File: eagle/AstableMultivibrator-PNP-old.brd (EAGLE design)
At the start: 30.5 x 15.2 mm, 10 parts, among them T1 BC557, T2 BC557

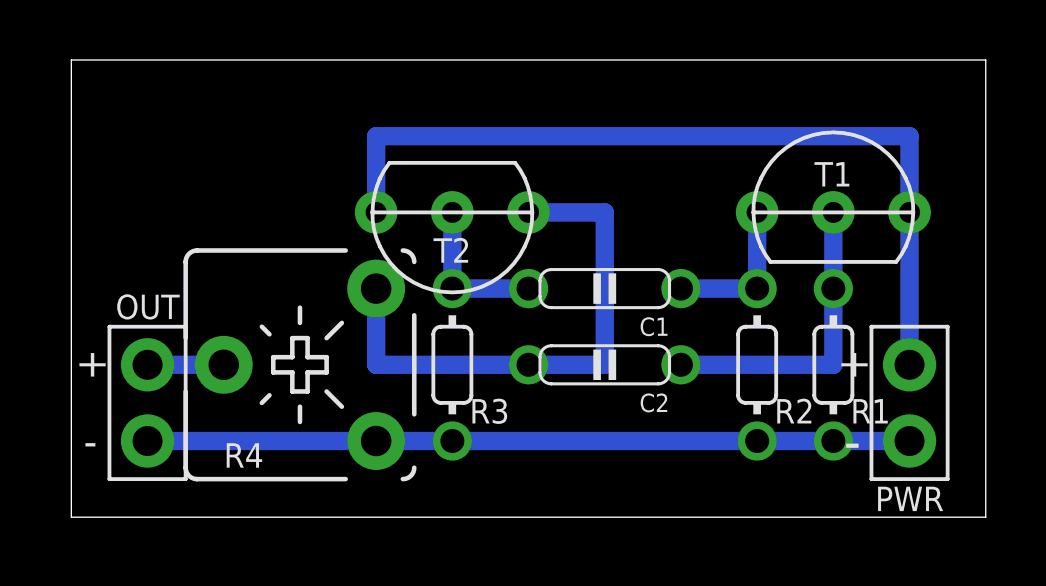
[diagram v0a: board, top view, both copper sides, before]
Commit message: ...
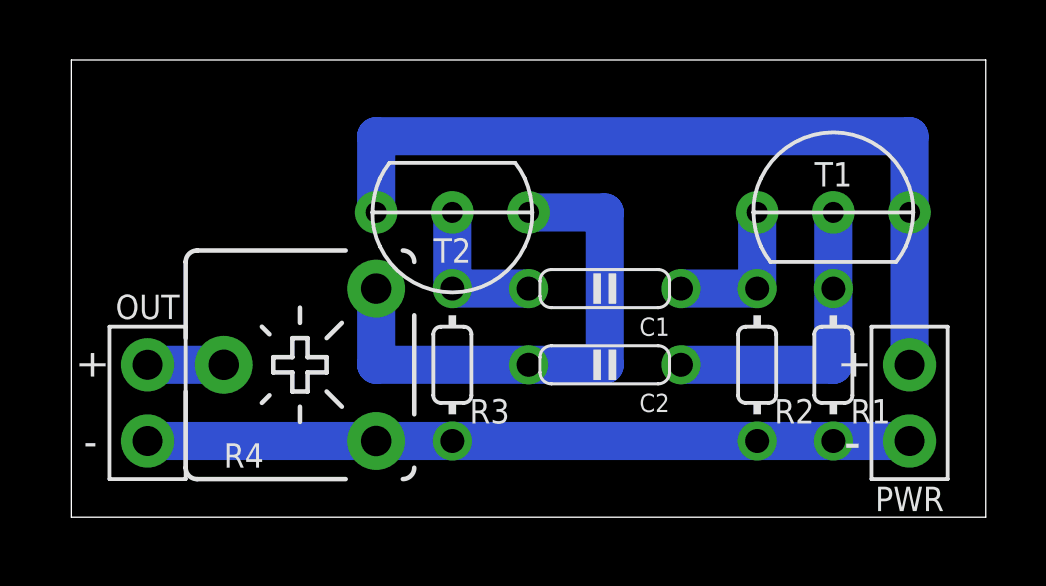
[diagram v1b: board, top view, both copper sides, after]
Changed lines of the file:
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@@
 <contactref element="C1" pad="1"/>
 <contactref element="R2" pad="2"/>
-<wire x1="20.32" y1="7.62" x2="22.86" y2="7.62" width="0.6096" layer="16"/>
-<wire x1="22.86" y1="7.62" x2="22.86" y2="10.16" width="0.6096" layer="16"/>
+<wire x1="20.32" y1="7.62" x2="22.86" y2="7.62" width="1.27" layer="16"/>
+<wire x1="22.86" y1="7.62" x2="22.86" y2="10.16" width="1.27" layer="16"/>
 <wire x1="22.86" y1="10.16" x2="22.86" y2="7.62" width="0" layer="19" extent="1-1"/>
 </signal>
@@
 <contactref element="C1" pad="2"/>
 <contactref element="R3" pad="2"/>
-<wire x1="15.24" y1="7.62" x2="12.7" y2="7.62" width="0.6096" layer="16"/>
-<wire x1="12.7" y1="7.62" x2="12.7" y2="10.16" width="0.6096" layer="16"/>
+<wire x1="15.24" y1="7.62" x2="12.7" y2="7.62" width="1.27" layer="16"/>
+<wire x1="12.7" y1="7.62" x2="12.7" y2="10.16" width="1.27" layer="16"/>
 </signal>
 <signal name="N$1">
@@
 <contactref element="C2" pad="2"/>
 <contactref element="R4" pad="E"/>
-<wire x1="15.24" y1="5.08" x2="10.16" y2="5.08" width="0.6096" layer="16"/>
-<wire x1="10.16" y1="5.08" x2="10.16" y2="7.62" width="0.6096" layer="16"/>
-<wire x1="15.24" y1="10.16" x2="17.78" y2="10.16" width="0.6096" layer="16"/>
-<wire x1="17.78" y1="10.16" x2="17.78" y2="5.08" width="0.6096" layer="16"/>
-<wire x1="17.78" y1="5.08" x2="15.24" y2="5.08" width="0.6096" layer="16"/>
+<wire x1="15.24" y1="5.08" x2="10.16" y2="5.08" width="1.27" layer="16"/>
+<wire x1="10.16" y1="5.08" x2="10.16" y2="7.62" width="1.27" layer="16"/>
+<wire x1="15.24" y1="10.16" x2="17.78" y2="10.16" width="1.27" layer="16"/>
+<wire x1="17.78" y1="10.16" x2="17.78" y2="5.08" width="1.27" layer="16"/>
+<wire x1="17.78" y1="5.08" x2="15.24" y2="5.08" width="1.27" layer="16"/>
 </signal>
 <signal name="N$3">
@@
 <contactref element="R1" pad="2"/>
 <via x="25.4" y="7.62" extent="1-16" drill="0.6" shape="square"/>
-<wire x1="20.32" y1="5.08" x2="25.4" y2="5.08" width="0.6096" layer="16"/>
-<wire x1="25.4" y1="5.08" x2="25.4" y2="10.16" width="0.6096" layer="16"/>
+<wire x1="20.32" y1="5.08" x2="25.4" y2="5.08" width="1.27" layer="16"/>
+<wire x1="25.4" y1="5.08" x2="25.4" y2="10.16" width="1.27" layer="16"/>
 <wire x1="25.4" y1="10.16" x2="25.4" y2="7.62" width="0" layer="19" extent="1-1"/>
 </signal>
@@
 <contactref element="OUT" pad="2"/>
 <contactref element="R4" pad="S"/>
-<wire x1="2.54" y1="5.08" x2="5.08" y2="5.08" width="0.6096" layer="16"/>
+<wire x1="2.54" y1="5.08" x2="5.08" y2="5.08" width="1.27" layer="16"/>
 </signal>
 <signal name="GND">
@@
 <contactref element="R3" pad="1"/>
 <contactref element="R1" pad="1"/>
-<wire x1="12.7" y1="2.54" x2="22.86" y2="2.54" width="0.6096" layer="16"/>
+<wire x1="12.7" y1="2.54" x2="22.86" y2="2.54" width="1.27" layer="16"/>
 <contactref element="J1" pad="1"/>
 <contactref element="OUT" pad="1"/>
-<wire x1="22.86" y1="2.54" x2="25.4" y2="2.54" width="0.6096" layer="16"/>
-<wire x1="27.94" y1="2.54" x2="25.4" y2="2.54" width="0.6096" layer="16"/>
+<wire x1="22.86" y1="2.54" x2="25.4" y2="2.54" width="1.27" layer="16"/>
+<wire x1="27.94" y1="2.54" x2="25.4" y2="2.54" width="1.27" layer="16"/>
 <contactref element="R4" pad="A"/>
-<wire x1="12.7" y1="2.54" x2="10.16" y2="2.54" width="0.6096" layer="16"/>
-<wire x1="2.54" y1="2.54" x2="10.16" y2="2.54" width="0.6096" layer="16"/>
+<wire x1="12.7" y1="2.54" x2="10.16" y2="2.54" width="1.27" layer="16"/>
+<wire x1="2.54" y1="2.54" x2="10.16" y2="2.54" width="1.27" layer="16"/>
 </signal>
 <signal name="VCC">
@@
 <contactref element="T2" pad="E"/>
 <contactref element="J1" pad="2"/>
-<wire x1="10.16" y1="10.16" x2="10.16" y2="12.7" width="0.6096" layer="16"/>
-<wire x1="10.16" y1="12.7" x2="27.94" y2="12.7" width="0.6096" layer="16"/>
-<wire x1="27.94" y1="12.7" x2="27.94" y2="10.16" width="0.6096" layer="16"/>
-<wire x1="27.94" y1="10.16" x2="27.94" y2="5.08" width="0.6096" layer="16"/>
+<wire x1="10.16" y1="10.16" x2="10.16" y2="12.7" width="1.27" layer="16"/>
+<wire x1="10.16" y1="12.7" x2="27.94" y2="12.7" width="1.27" layer="16"/>
+<wire x1="27.94" y1="12.7" x2="27.94" y2="10.16" width="1.27" layer="16"/>
+<wire x1="27.94" y1="10.16" x2="27.94" y2="5.08" width="1.27" layer="16"/>
 </signal>
 </signals>
